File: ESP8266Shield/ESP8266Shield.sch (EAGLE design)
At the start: 19 parts, among them IC1 MEGA8-P, Q1 2N5088, Q2 2N5088

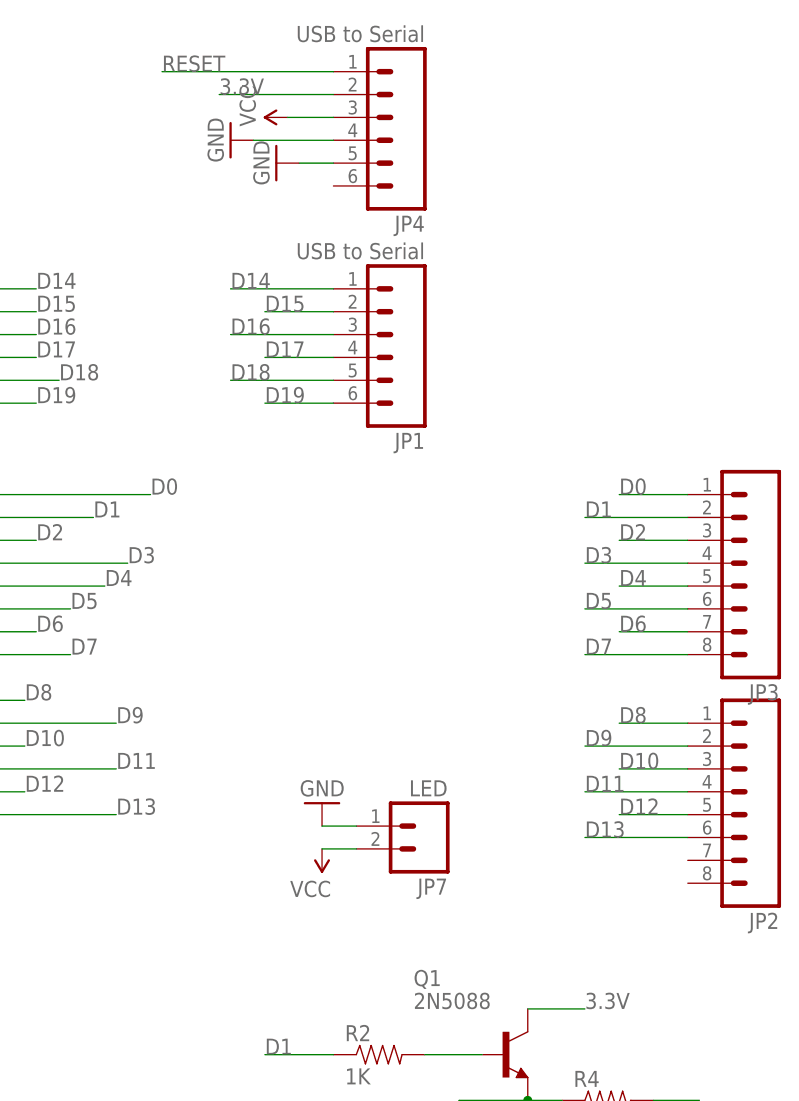
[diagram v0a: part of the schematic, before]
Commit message: v0.06
Added Shield schematic, and gerber files.
It has not yet been verified.
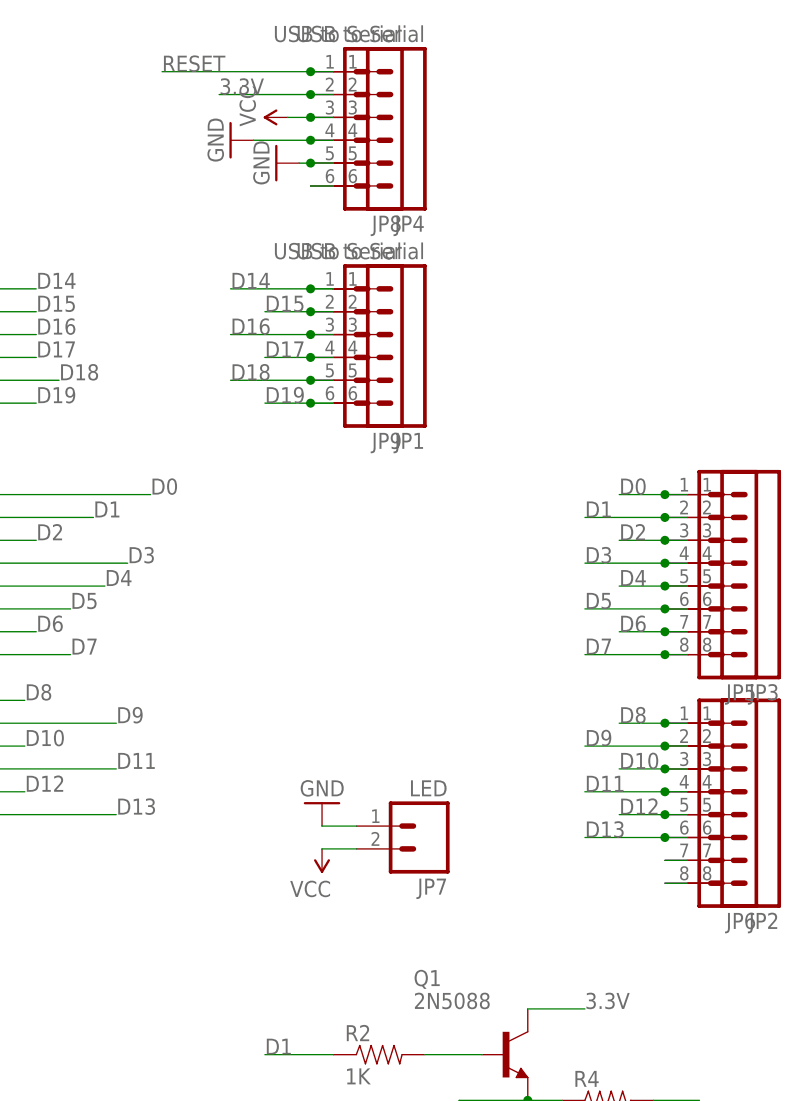
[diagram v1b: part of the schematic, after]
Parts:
- added JP5, JP6: (no value), SparkFun:M08
- added JP8, JP9: USB to Serial, SparkFun:M06SIP
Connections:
- new net N$5: JP2.7, JP6.7
- new net N$6: JP2.8, JP6.8
- new net N$7: JP4.6, JP8.6
- net 3.3V: now also JP8.2
- net D0: now also JP5.1
- net D1: now also JP5.2
- net D10: now also JP6.3
- net D11: now also JP6.4
- net D12: now also JP6.5
- net D13: now also JP6.6
- net D14: now also JP9.1
- net D15: now also JP9.2
- net D16: now also JP9.3
- net D17: now also JP9.4
- net D18: now also JP9.5
- net D19: now also JP9.6
- net D2: now also JP5.3
- net D3: now also JP5.4
- net D4: now also JP5.5
- net D5: now also JP5.6
- net D6: now also JP5.7
- net D7: now also JP5.8
- net D8: now also JP6.1
- net D9: now also JP6.2
- net GND: now also JP8.4, JP8.5
- net RESET: now also JP8.1
- net VCC: now also JP8.3
